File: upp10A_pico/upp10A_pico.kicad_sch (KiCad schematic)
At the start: 75 parts, among them J10 Conn_01x07, J11 Conn_01x03, J3 Conn_01x03, J4 Conn_01x03, J5 Conn_01x05, J6 Conn_01x05, J7 Conn_01x05, J8 Conn_01x05, J9 Conn_01x03, Q1 BF545A, Q2 BF545A, Q3 BF545A, Q4 RK7002, Q5 RK7002, Q6 RK7002, Q7 RK7002, U1 4555, U2 4052, U3 4013, U4 MAX3232, U5 OP07, U6 ICL7660, U7 RPi PICO

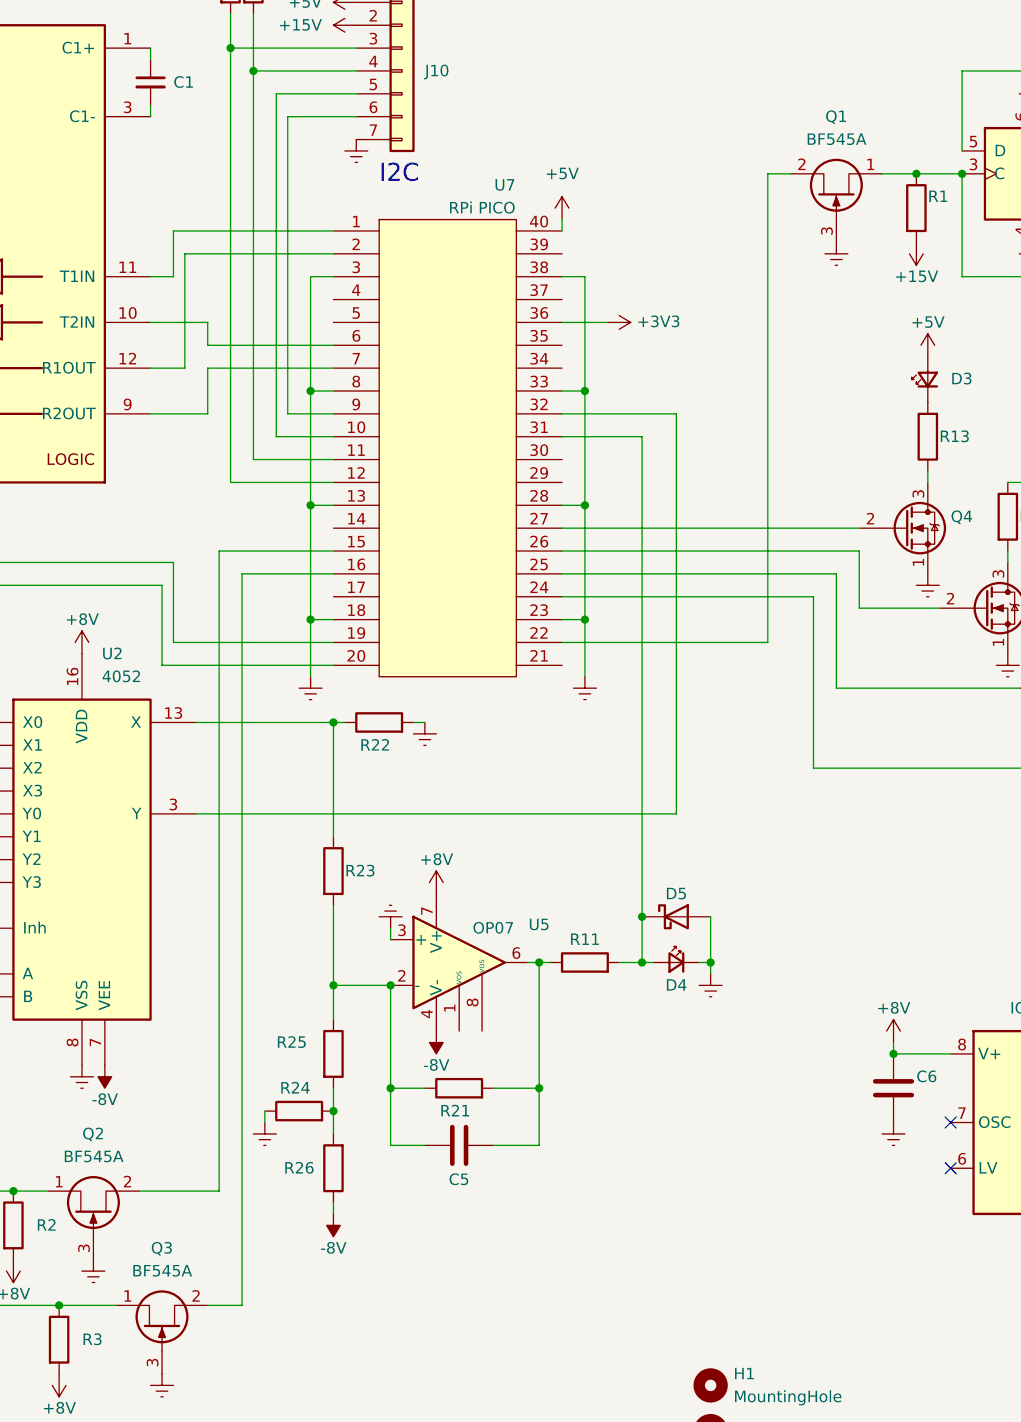
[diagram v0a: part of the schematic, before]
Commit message: Made corrections on PCB; added gerber files; added schematic in pdf;
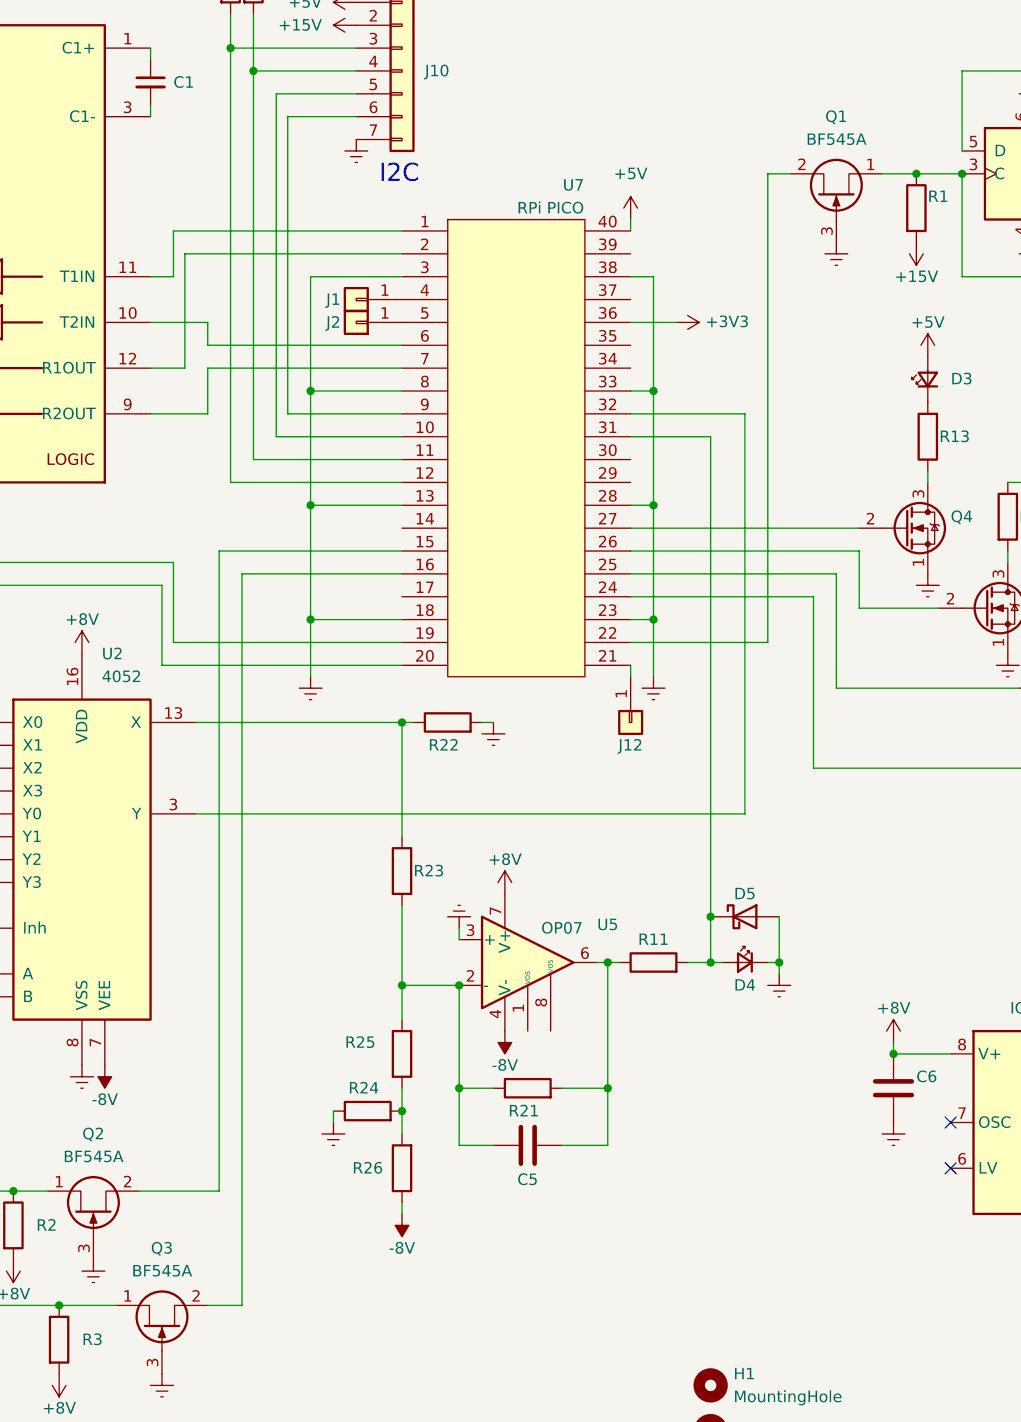
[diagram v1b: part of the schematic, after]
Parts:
- added J1, J12, J2: Conn_01x01, Connector_Pin:Pin_D1.0mm_L10.0mm, symbol Connector_Generic:Conn_01x01
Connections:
- net at U7.21: now also J12.1 (Pin_1)
- net at U7.4: now also J1.1 (Pin_1)
- net at U7.5: now also J2.1 (Pin_1)
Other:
- moved on the sheet: C5, D4, D5, R11, R21, R22, R23, R24, R25, R26, U5, U7
